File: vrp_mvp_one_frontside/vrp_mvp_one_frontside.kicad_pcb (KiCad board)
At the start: 2 copper layers, 77 x 150 mm, 88 parts, among them J1 Micro_SD_Card, J2 BACKSIDE_INTERFACE_1, J4 USB_C_Receptacle_USB2.0_16P, J6 DEBUG, J7 BACKSIDE_INTERFACE_2, J8 SJ3-35094BG, Q1 MMBT2222A, Q2 MMBT2222A, Q3 MMBT2222A, SW1 SEND, SW10 TWO, SW11 THREE, SW12 FOUR, SW13 FIVE, SW14 SIX, SW15 SEVEN, SW16 EIGHT, SW17 NINE, SW18 ALPHA, SW19 BETA, SW2 END, SW20 ZERO, SW21 RESET, SW3 PAGE, SW4 CLR, SW5 POUND, SW6 UP, SW7 DOWN, SW8 ASTERISK, SW9 ONE, U2 NHD-C0220BIZ, U3 ATSAMD21G18A-A, U4 TLV320AIC3104IRHBT, U5 SN74CB3Q3257PWR

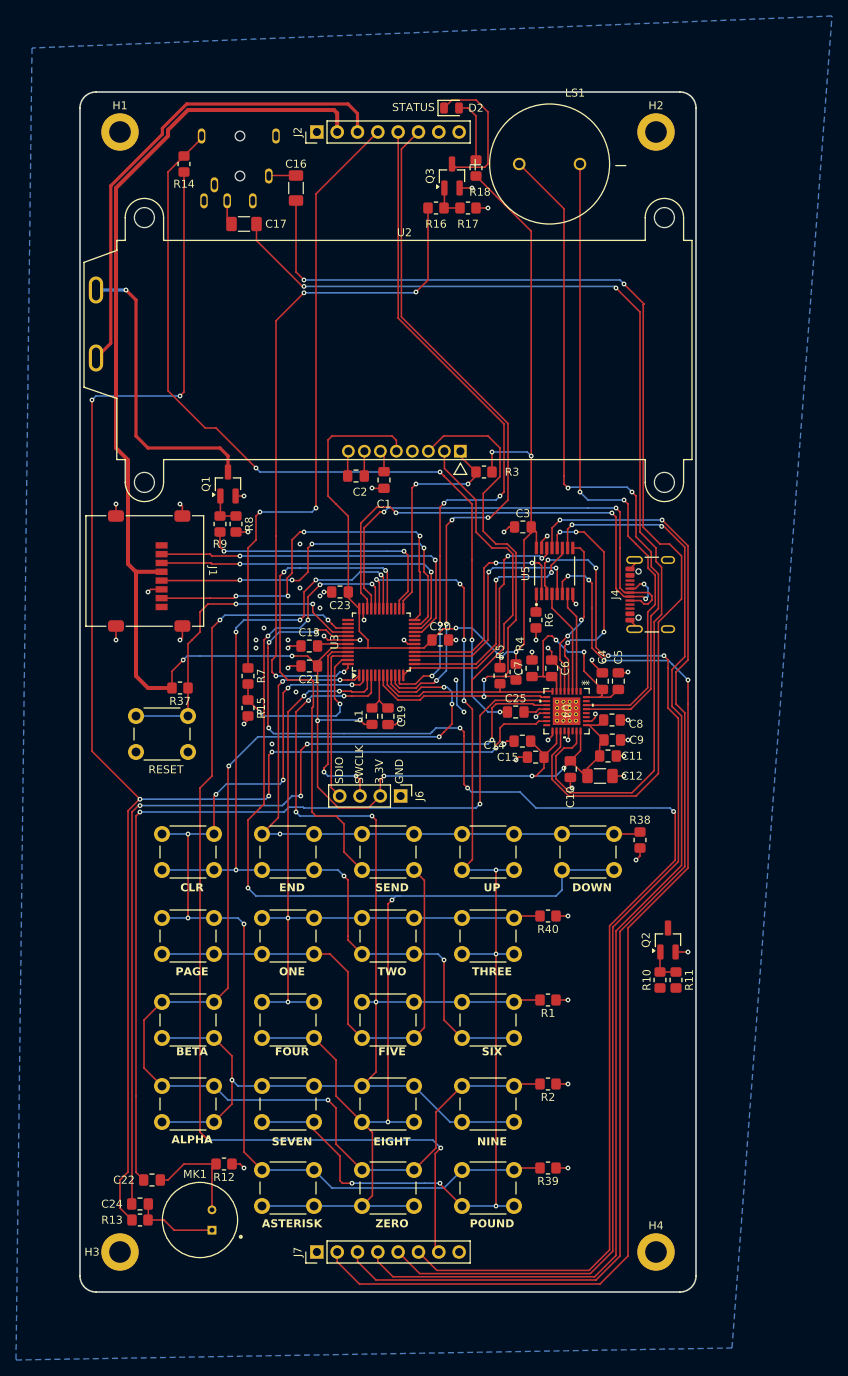
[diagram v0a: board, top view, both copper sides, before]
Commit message: response to issue 1
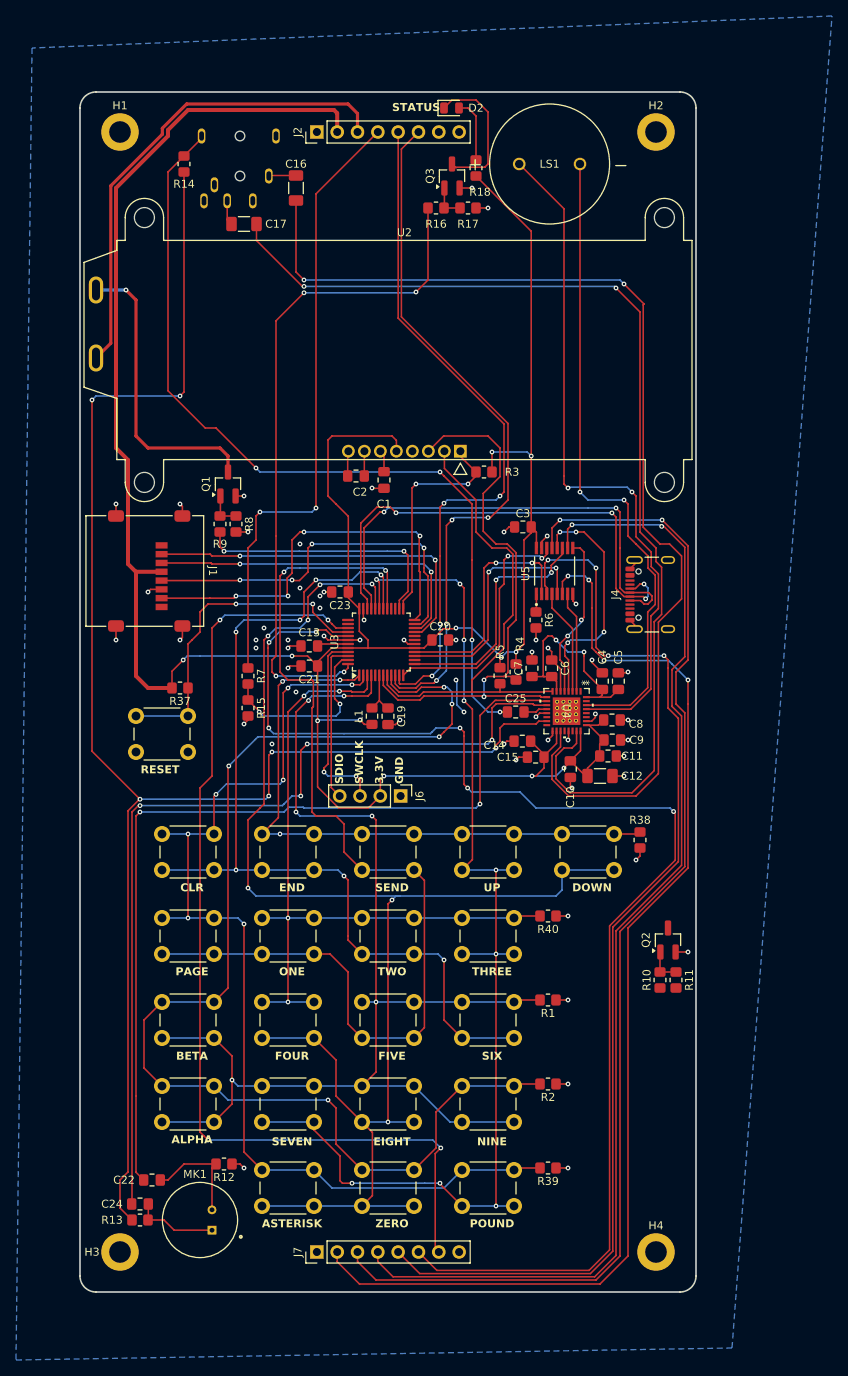
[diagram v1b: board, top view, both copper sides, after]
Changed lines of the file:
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@@
 		(property "Value" "SEND"
 			(at 3.75 6.7 0)
-			(layer "F.SilkS")
+			(layer "F.SilkS" knockout)
 			(effects
 				(font
@@
 		(property "Value" "PAGE"
 			(at 3.75 6.7 0)
-			(layer "F.SilkS")
+			(layer "F.SilkS" knockout)
 			(effects
 				(font
@@
 		)
 		(property "Value" "SIX"
-			(at 3.75 6.2 0)
-			(layer "F.SilkS")
+			(at 3.75 6.75 0)
+			(layer "F.SilkS" knockout)
 			(effects
 				(font
@@
 		(property "Value" "EIGHT"
 			(at 3.75 6.95 0)
-			(layer "F.SilkS")
+			(layer "F.SilkS" knockout)
 			(effects
 				(font
@@
 		(property "Value" "TWO"
 			(at 3.75 6.7 0)
-			(layer "F.SilkS")
+			(layer "F.SilkS" knockout)
 			(effects
 				(font
@@
 		(property "Value" "END"
 			(at 3.75 6.7 0)
-			(layer "F.SilkS")
+			(layer "F.SilkS" knockout)
 			(effects
 				(font
@@
 		(property "Value" "ALPHA"
 			(at 3.75 6.7 0)
-			(layer "F.SilkS")
+			(layer "F.SilkS" knockout)
 			(effects
 				(font
@@
 		(at 121.7 29)
 		(property "Reference" "LS1"
-			(at 3.175 -8.885 0)
+			(at 0 0 0)
 			(layer "F.SilkS")
 			(effects
@@
 		(property "Value" "ZERO"
 			(at 3.75 6.7 0)
-			(layer "F.SilkS")
+			(layer "F.SilkS" knockout)
 			(effects
 				(font
@@
 		(property "Value" "UP"
 			(at 3.75 6.7 0)
-			(layer "F.SilkS")
+			(layer "F.SilkS" knockout)
 			(effects
 				(font
@@
 		(property "Value" "CLR"
 			(at 3.75 6.7 0)
-			(layer "F.SilkS")
+			(layer "F.SilkS" knockout)
 			(effects
 				(font
@@
 		)
 		(property "Value" "RESET"
-			(at 3.75 6.7 0)
-			(layer "F.SilkS")
+			(at 3 6.7 0)
+			(layer "F.SilkS" knockout)
 			(effects
 				(font
 					(size 1 1)
-					(thickness 0.15)
+					(thickness 0.2)
+					(bold yes)
 				)
 			)
@@
 		)
 		(property "Value" "BETA"
-			(at 3.75 6.2 0)
-			(layer "F.SilkS")
+			(at 3.75 6.75 0)
+			(layer "F.SilkS" knockout)
 			(effects
 				(font
@@
 		(property "Value" "NINE"
 			(at 3.75 6.95 0)
-			(layer "F.SilkS")
+			(layer "F.SilkS" knockout)
 			(effects
 				(font
@@
 		(property "Value" "SEVEN"
 			(at 3.75 6.95 0)
-			(layer "F.SilkS")
+			(layer "F.SilkS" knockout)
 			(effects
 				(font
@@
 		(property "Value" "POUND"
 			(at 3.75 6.7 0)
-			(layer "F.SilkS")
+			(layer "F.SilkS" knockout)
 			(effects
 				(font
@@
 		)
 		(property "Value" "FOUR"
-			(at 3.75 6.2 0)
-			(layer "F.SilkS")
+			(at 3.75 6.75 0)
+			(layer "F.SilkS" knockout)
 			(effects
 				(font
@@
 		)
 		(property "Value" "FIVE"
-			(at 3.75 6.2 0)
-			(layer "F.SilkS")
+			(at 3.75 6.75 0)
+			(layer "F.SilkS" knockout)
 			(effects
 				(font
@@
 		(property "Value" "ASTERISK"
 			(at 3.75 6.7 0)
-			(layer "F.SilkS")
+			(layer "F.SilkS" knockout)
 			(effects
 				(font
@@
 		(property "Value" "DOWN"
 			(at 3.75 6.7 0)
-			(layer "F.SilkS")
+			(layer "F.SilkS" knockout)
 			(effects
 				(font
@@
 		(property "Value" "THREE"
 			(at 3.75 6.7 0)
-			(layer "F.SilkS")
+			(layer "F.SilkS" knockout)
 			(effects
 				(font
@@
 		(property "Value" "ONE"
 			(at 3.75 6.7 0)
-			(layer "F.SilkS")
+			(layer "F.SilkS" knockout)
 			(effects
 				(font
@@
 	(gr_text "GND"
 		(at 103.5 106.5 90)
-		(layer "F.SilkS")
+		(layer "F.SilkS" knockout)
 		(effects
 			(font
 				(size 1 1)
-				(thickness 0.125)
+				(thickness 0.2)
+				(bold yes)
 			)
 			(justify left bottom)
@@
 	(gr_text "STATUS"
 		(at 102 22.5 0)
-		(layer "F.SilkS")
+		(layer "F.SilkS" knockout)
 		(effects
 			(font
 				(size 1 1)
-				(thickness 0.125)
+				(thickness 0.2)
+				(bold yes)
 			)
 			(justify left bottom)
@@
 	(gr_text "SDIO"
 		(at 96 106.5 90)
-		(layer "F.SilkS")
+		(layer "F.SilkS" knockout)
 		(effects
 			(font
 				(size 1 1)
-				(thickness 0.125)
+				(thickness 0.2)
+				(bold yes)
 			)
 			(justify left bottom)
@@
 	(gr_text "3.3V"
 		(at 101 106.5 90)
-		(layer "F.SilkS")
+		(layer "F.SilkS" knockout)
 		(effects
 			(font
 				(size 1 1)
-				(thickness 0.125)
+				(thickness 0.2)
+				(bold yes)
 			)
 			(justify left bottom)
@@
 	(gr_text "SWCLK"
 		(at 98.5 106.5 90)
-		(layer "F.SilkS")
+		(layer "F.SilkS" knockout)
 		(effects
 			(font
 				(size 1 1)
-				(thickness 0.125)
+				(thickness 0.2)
+				(bold yes)
 			)
 			(justify left bottom)
